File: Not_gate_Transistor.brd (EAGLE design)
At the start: 24.3 x 22.9 mm, 8 parts, among them Q1 BC547A

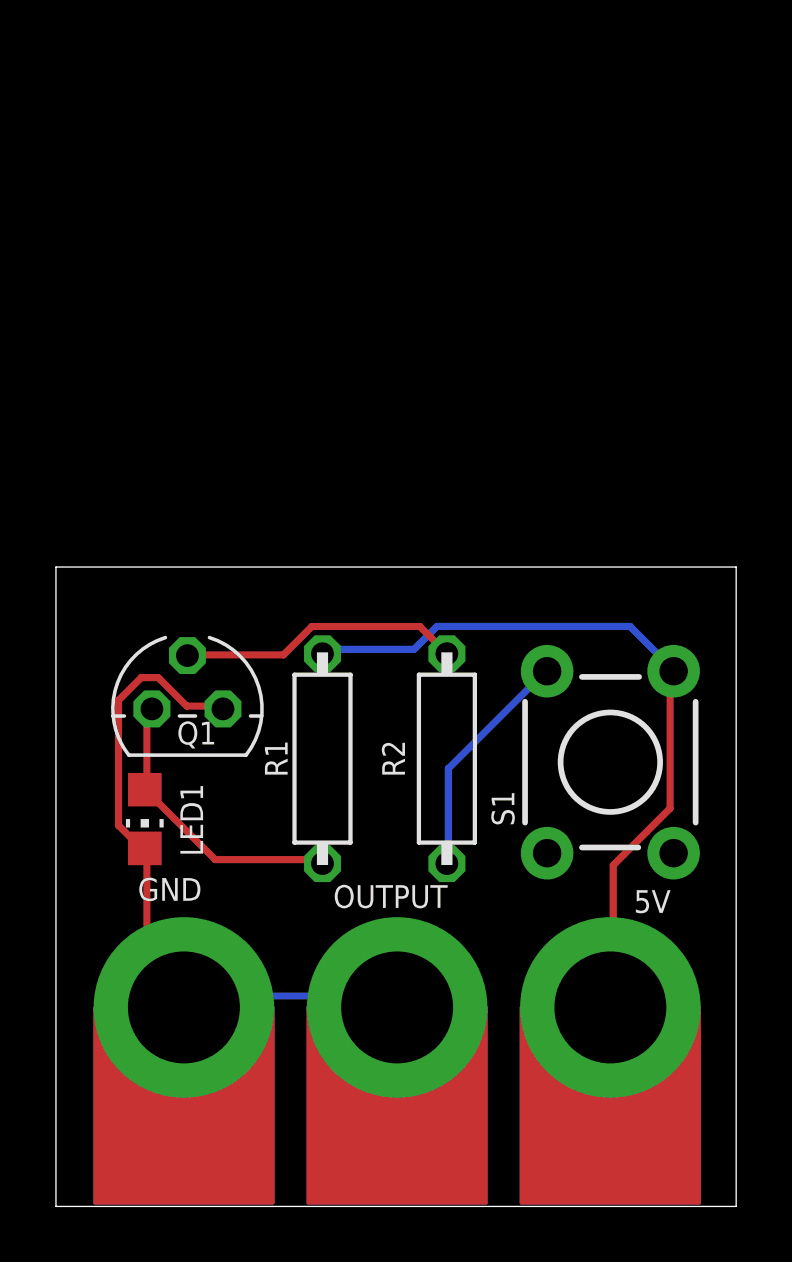
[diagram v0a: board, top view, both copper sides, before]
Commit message: update
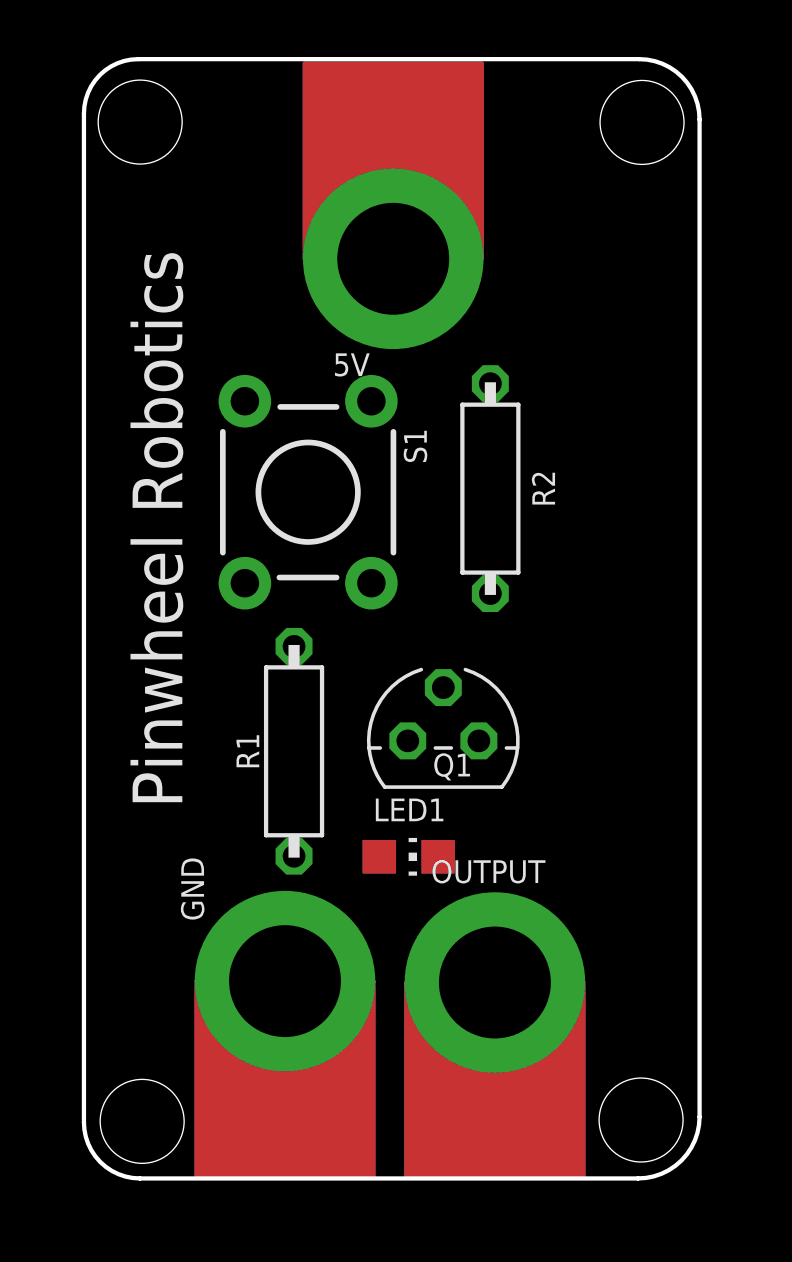
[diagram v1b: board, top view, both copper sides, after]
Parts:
- moved 5V 27.9 mm to (12.1, 33.9), turned to 180 degrees
- moved S1 14.5 mm to (9.01, 25.5), turned to 90 degrees
- moved R2 9.77 mm to (15.5, 25.7), turned to 270 degrees
- moved LED1 9.52 mm to (12.6, 12.5), turned to 270 degrees
- moved Q1 9.22 mm to (13.8, 16.6)
- moved GND 3.73 mm to (8.19, 8.05)
- moved OUTPUT 3.61 mm to (15.7, 8.00)
- moved R1 1.05 mm to (8.51, 16.3)
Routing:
- net 5V: track 26.8 -> 0.00 mm
- net GND: track 24.5 -> 0.00 mm
- net N$2: track 10.4 -> 0.00 mm
- net N$3: track 10.1 -> 0.00 mm
- net N$4: track 8.37 -> 0.00 mm
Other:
- board size 24.3 x 22.9 mm -> 22 x 40 mm
- board text added: "Pinwheel Robotics"
- board text added: "care@pinwheel.in"

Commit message: New Updates
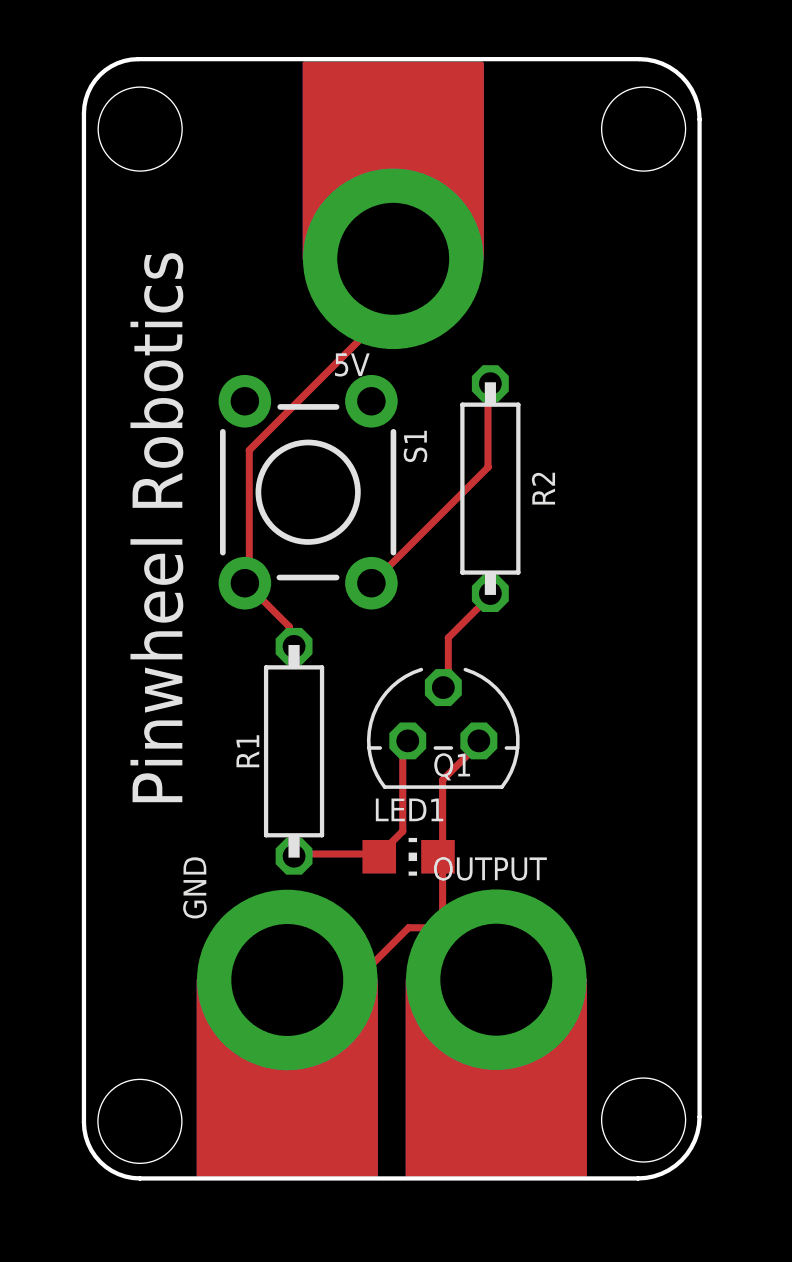
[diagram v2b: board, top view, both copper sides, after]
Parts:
- moved OUTPUT 0.11 mm to (15.7, 8.10)
- moved GND 0.09 mm to (8.27, 8.09)
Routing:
- net GND: track 0.00 -> 19.1 mm
- net 5V: track 0.00 -> 16.8 mm
- net N$4: track 0.00 -> 8.89 mm
- net N$2: track 0.00 -> 7.69 mm
- net N$3: track 0.00 -> 4.05 mm
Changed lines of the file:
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@@
 <drawing>
 <settings>
-<setting alwaysvectorfont="yes"/>
+<setting alwaysvectorfont="no"/>
 <setting verticaltext="up"/>
 </settings>
@@
 <plain>
 <text x="4.516" y="14.23" size="1.778" layer="21" rot="R90">Pinwheel Robotics </text>
-<hole x="3.009" y="38.751" drill="3"/>
-<hole x="20.944" y="38.738" drill="3"/>
-<hole x="3.08" y="3.04" drill="3"/>
-<hole x="20.91" y="3.088" drill="3"/>
+<hole x="3.009" y="38.5" drill="3"/>
+<hole x="21" y="38.5" drill="3"/>
+<hole x="3" y="3.04" drill="3"/>
+<hole x="21" y="3.088" drill="3"/>
 <wire x1="1" y1="39.059846875" x2="1" y2="3.00098125" width="0.1524" layer="20"/>
 <wire x1="1" y1="3.00098125" x2="3.00098125" y2="1" width="0.1524" layer="20" curve="90"/>
@@
 <attribute name="NAME" x="9.894" y="29.673" size="0.8128" layer="21" font="vector"/>
 </element>
-<element name="GND" library="microbit" package="MICROBIT_PAD" value="MICROBIT_PAD" x="8.185" y="8.052" smashed="yes">
-<attribute name="NAME" x="5.291" y="10.194" size="0.8128" layer="21" font="vector" rot="R90"/>
+<element name="GND" library="microbit" package="MICROBIT_PAD" value="MICROBIT_PAD" x="8.266084375" y="8.092525" smashed="yes">
+<attribute name="NAME" x="5.372084375" y="10.234525" size="0.8128" layer="21" font="vector" rot="R90"/>
 </element>
 <element name="LED1" library="led" library_urn="urn:adsk.eagle:library:259" package="CHIP-LED0805" package3d_urn="urn:adsk.eagle:package:15818/2" value="" x="12.603" y="12.494" smashed="yes" rot="R270">
@@
 <attribute name="VALUE" x="11.333" y="9.954" size="1.27" layer="27"/>
 </element>
-<element name="OUTPUT" library="microbit" package="MICROBIT_PAD" value="MICROBIT_PAD" x="15.686" y="8.002" smashed="yes">
-<attribute name="NAME" x="13.4" y="11.558" size="0.8128" layer="21" font="vector"/>
+<element name="OUTPUT" library="microbit" package="MICROBIT_PAD" value="MICROBIT_PAD" x="15.73645625" y="8.102915625" smashed="yes">
+<attribute name="NAME" x="13.45045625" y="11.658915625" size="0.8128" layer="21" font="vector"/>
 </element>
 <element name="Q1" library="transistor-npn" library_urn="urn:adsk.eagle:library:398" package="TO92" package3d_urn="urn:adsk.eagle:package:28523/2" value="BC547A" x="13.843" y="16.637" smashed="yes">
@@
 <contactref element="OUTPUT" pad="PAD"/>
 <contactref element="GND" pad="PAD"/>
-<wire x1="13.653" y1="12.494" x2="15.113" y2="16.637" width="0" layer="19" extent="1-1"/>
-<wire x1="8.185" y1="8.052" x2="13.653" y2="12.494" width="0" layer="19" extent="1-1"/>
-<wire x1="15.686" y1="8.002" x2="8.185" y2="8.052" width="0" layer="19" extent="1-1"/>
+<wire x1="13.8176" y1="15.24" x2="13.8176" y2="12.5984" width="0.254" layer="1"/>
+<wire x1="15.0368" y1="16.4592" x2="13.8176" y2="15.24" width="0.254" layer="1"/>
+<wire x1="13.8176" y1="12.5984" x2="13.653" y2="12.494" width="0.254" layer="1"/>
+<wire x1="15.0368" y1="16.4592" x2="15.113" y2="16.637" width="0.254" layer="1"/>
+<wire x1="13.8176" y1="9.9568" x2="13.8176" y2="12.3952" width="0.254" layer="1"/>
+<wire x1="15.6464" y1="8.128" x2="13.8176" y2="9.9568" width="0.254" layer="1"/>
+<wire x1="13.8176" y1="12.3952" x2="13.653" y2="12.494" width="0.254" layer="1"/>
+<wire x1="15.6464" y1="8.128" x2="15.73645625" y2="8.102915625" width="0.254" layer="1"/>
+<wire x1="10.7696" y1="8.128" x2="8.3312" y2="8.128" width="0.254" layer="1"/>
+<wire x1="12.5984" y1="9.9568" x2="10.7696" y2="8.128" width="0.254" layer="1"/>
+<wire x1="13.8176" y1="9.9568" x2="12.5984" y2="9.9568" width="0.254" layer="1"/>
+<wire x1="8.3312" y1="8.128" x2="8.266084375" y2="8.092525" width="0.254" layer="1"/>
+<wire x1="13.8176" y1="9.9568" x2="15.73645625" y2="8.102915625" width="0.254" layer="1"/>
 </signal>
 <signal name="N$2">
@@
 <contactref element="R1" pad="1"/>
 <contactref element="LED1" pad="A"/>
-<wire x1="11.553" y1="12.494" x2="12.573" y2="16.637" width="0" layer="19" extent="1-1"/>
-<wire x1="8.509" y1="12.514" x2="11.553" y2="12.494" width="0" layer="19" extent="1-1"/>
+<wire x1="8.5344" y1="12.5984" x2="11.3792" y2="12.5984" width="0.254" layer="1"/>
+<wire x1="11.3792" y1="12.5984" x2="11.553" y2="12.494" width="0.254" layer="1"/>
+<wire x1="8.5344" y1="12.5984" x2="8.509" y2="12.514" width="0.254" layer="1"/>
+<wire x1="12.3952" y1="13.4112" x2="12.3952" y2="16.4592" width="0.254" layer="1"/>
+<wire x1="11.5824" y1="12.5984" x2="12.3952" y2="13.4112" width="0.254" layer="1"/>
+<wire x1="12.3952" y1="16.4592" x2="12.573" y2="16.637" width="0.254" layer="1"/>
+<wire x1="11.5824" y1="12.5984" x2="11.553" y2="12.494" width="0.254" layer="1"/>
 </signal>
 <signal name="N$3">
 <contactref element="R2" pad="2"/>
 <contactref element="Q1" pad="2"/>
-<wire x1="13.843" y1="18.542" x2="15.524" y2="21.902" width="0" layer="19" extent="1-1"/>
+<wire x1="14.0208" y1="20.32" x2="14.0208" y2="18.6944" width="0.254" layer="1"/>
+<wire x1="15.4432" y1="21.7424" x2="14.0208" y2="20.32" width="0.254" layer="1"/>
+<wire x1="14.0208" y1="18.6944" x2="13.843" y2="18.542" width="0.254" layer="1"/>
+<wire x1="15.4432" y1="21.7424" x2="15.524" y2="21.902" width="0.254" layer="1"/>
 </signal>
 <signal name="N$4">
 <contactref element="S1" pad="3"/>
 <contactref element="R2" pad="1"/>
-<wire x1="15.524" y1="29.402" x2="11.2726" y2="22.2718" width="0" layer="19" extent="1-1"/>
+<wire x1="15.4432" y1="26.416" x2="15.4432" y2="29.2608" width="0.254" layer="1"/>
+<wire x1="11.3792" y1="22.352" x2="15.4432" y2="26.416" width="0.254" layer="1"/>
+<wire x1="15.4432" y1="29.2608" x2="15.524" y2="29.402" width="0.254" layer="1"/>
+<wire x1="11.3792" y1="22.352" x2="11.2726" y2="22.2718" width="0.254" layer="1"/>
 </signal>
 <signal name="5V">
@@
 <contactref element="5V" pad="PAD"/>
 <contactref element="R1" pad="2"/>
-<wire x1="8.509" y1="20.014" x2="6.7514" y2="22.2718" width="0" layer="19" extent="1-1"/>
-<wire x1="12.053" y1="33.864" x2="6.7514" y2="22.2718" width="0" layer="19" extent="1-1"/>
+<wire x1="8.3312" y1="20.7264" x2="8.3312" y2="20.1168" width="0.254" layer="1"/>
+<wire x1="6.9088" y1="22.1488" x2="8.3312" y2="20.7264" width="0.254" layer="1"/>
+<wire x1="8.3312" y1="20.1168" x2="8.509" y2="20.014" width="0.254" layer="1"/>
+<wire x1="6.9088" y1="22.1488" x2="6.7514" y2="22.2718" width="0.254" layer="1"/>
+<wire x1="6.9088" y1="27.0256" x2="6.9088" y2="22.352" width="0.254" layer="1"/>
+<wire x1="11.9888" y1="32.1056" x2="6.9088" y2="27.0256" width="0.254" layer="1"/>
+<wire x1="11.9888" y1="33.7312" x2="11.9888" y2="32.1056" width="0.254" layer="1"/>
+<wire x1="6.9088" y1="22.352" x2="6.7514" y2="22.2718" width="0.254" layer="1"/>
+<wire x1="11.9888" y1="33.7312" x2="12.053" y2="33.864" width="0.254" layer="1"/>
 </signal>
 </signals>
